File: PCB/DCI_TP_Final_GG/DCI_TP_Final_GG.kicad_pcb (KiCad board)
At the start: 2 copper layers, 42 x 90 mm, 69 parts, among them J201 DRIVER A OUT, J301 DRIVER B OUT, J401 IN - Driver A, J402 IN - Driver B, J403 Vin, J404 Vout, U201 A3967, U301 A3967, U401 LM317

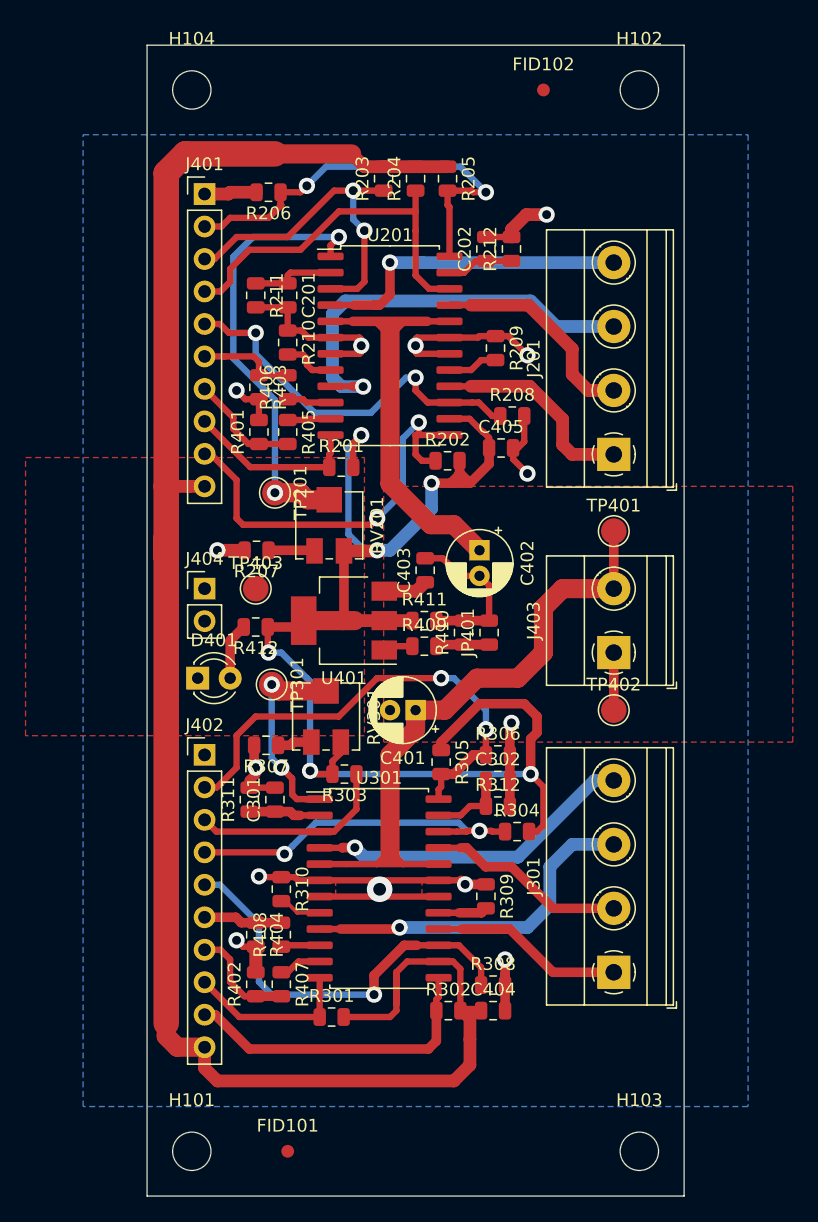
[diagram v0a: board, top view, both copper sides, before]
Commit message: Avance en Routeo
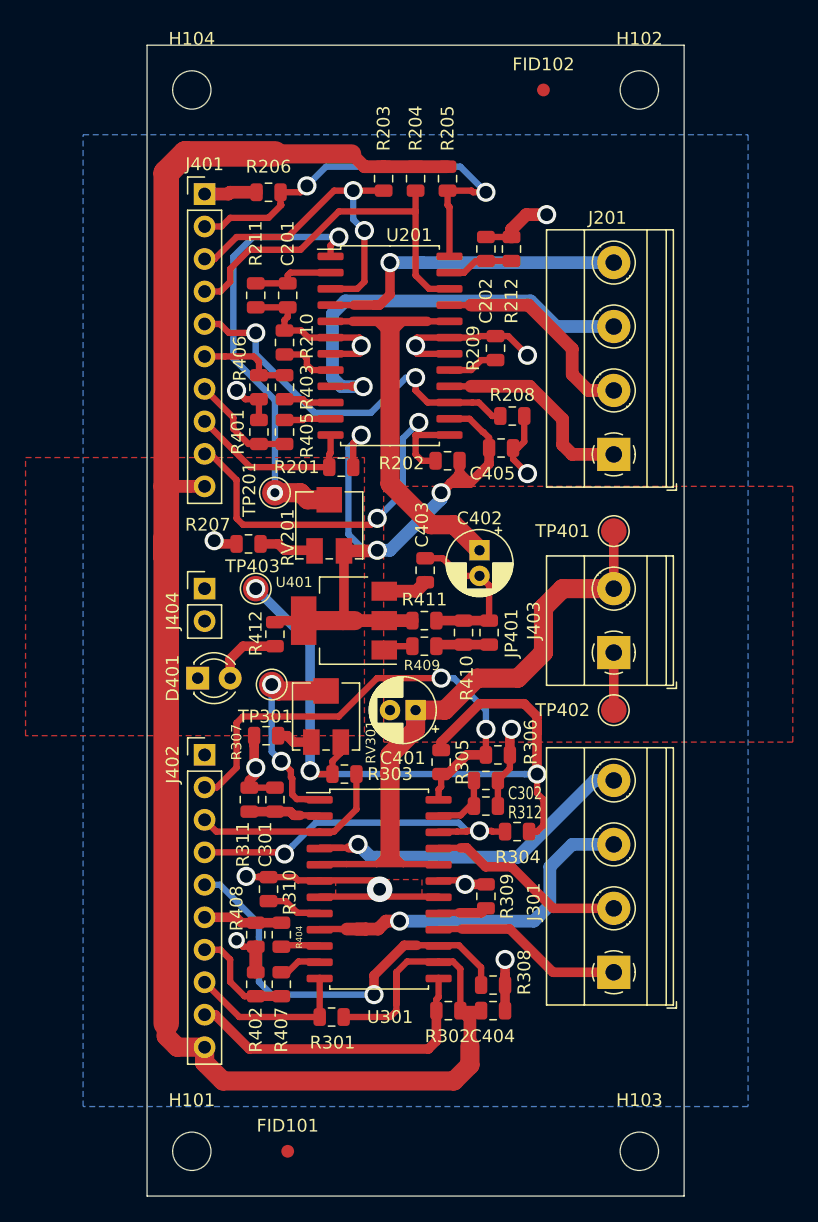
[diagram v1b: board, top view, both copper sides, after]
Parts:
- moved R412 1.60 mm to (116.5, 96.6), turned to 270 degrees
- moved R310 1.00 mm to (116.0, 116.5)
- moved C302 0.94 mm to (133.0, 108.0)
- moved R312 0.94 mm to (133.0, 110.0)
- moved R207 0.80 mm to (114.4, 89.5)
- moved R307 0.75 mm to (115.8, 104.5)
- moved R210 0.25 mm to (117.2, 73.8)
- moved R405 0.25 mm to (117.2, 80.8)
- moved R406 0.25 mm to (117.2, 77.2)
- moved U301 0.06 mm to (124.7, 116.5)
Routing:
- net VCC: track 257.4 -> 268.3 mm
- net GND: track 114.7 -> 111.8 mm
- net /Driver B/DB-O2B: track 25.8 -> 27.8 mm
- net Net-(R310-Pad2): track 3.04 -> 4.38 mm
- net Net-(C302-Pad1): track 6.00 -> 4.75 mm
- net Net-(D401-Pad2): track 4.44 -> 5.41 mm
- net Net-(R207-Pad1): track 3.62 -> 4.45 mm
- net /Driver B/PFD-B: track 37.7 -> 38.3 mm
